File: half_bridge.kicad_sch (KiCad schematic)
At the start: 18 parts, among them Q1 60V 95A, Q2 60V 95A

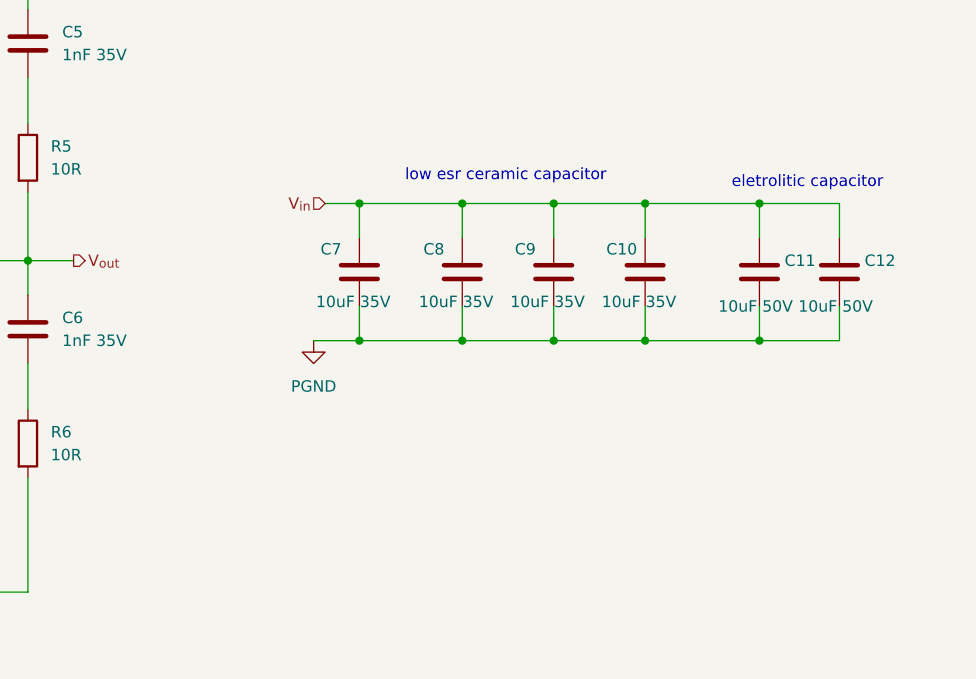
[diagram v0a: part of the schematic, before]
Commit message: added wire step
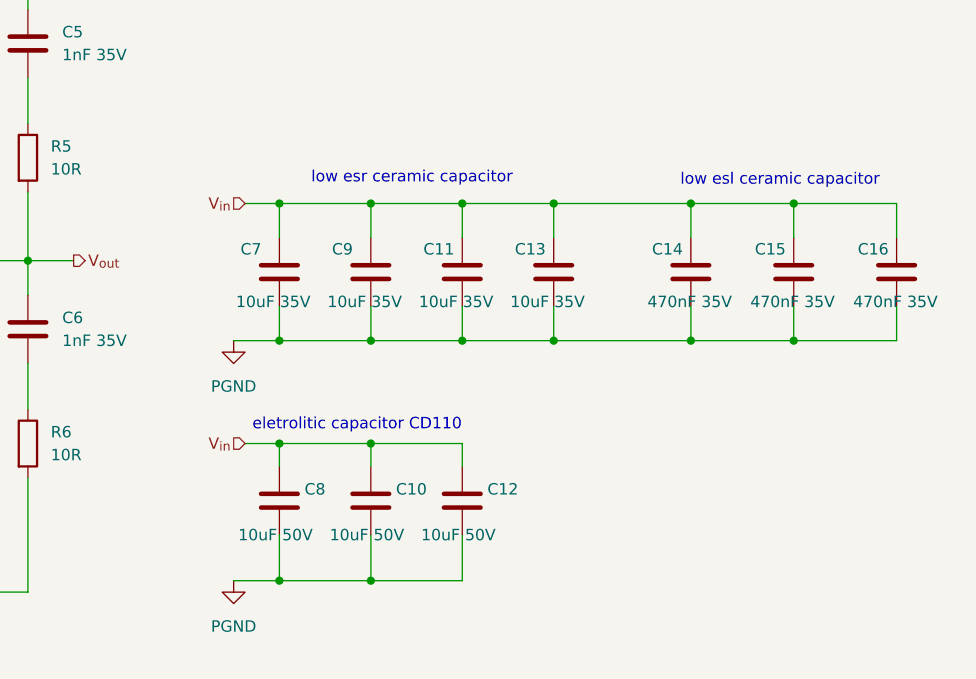
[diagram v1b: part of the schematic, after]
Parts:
- added C12: 10uF 50V, Capacitor_THT:C_Radial_D5.0mm_H11.0mm_P2.00mm, symbol Device:C
- added C14, C15, C16: 470nF 35V, Capacitor_SMD:C_0603_1608Metric, symbol Device:C
- renumbered C12 to C10, C9 to C11, C10 to C13, C11 to C8, C8 to C9
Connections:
- net PGND: now also C12.2, C14.2, C15.2, C16.2
- net V_{in}: now also C12.1, C14.1, C15.1, C16.1
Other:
- note added: "eletrolitic capacitor CD110"
- note added: "low esl ceramic capacitor"
- note removed: "eletrolitic capacitor"
- moved on the sheet: C10, C11, C13, C7, C8, C9
